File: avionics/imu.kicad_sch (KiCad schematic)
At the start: 3 parts, among them U2 BMI088

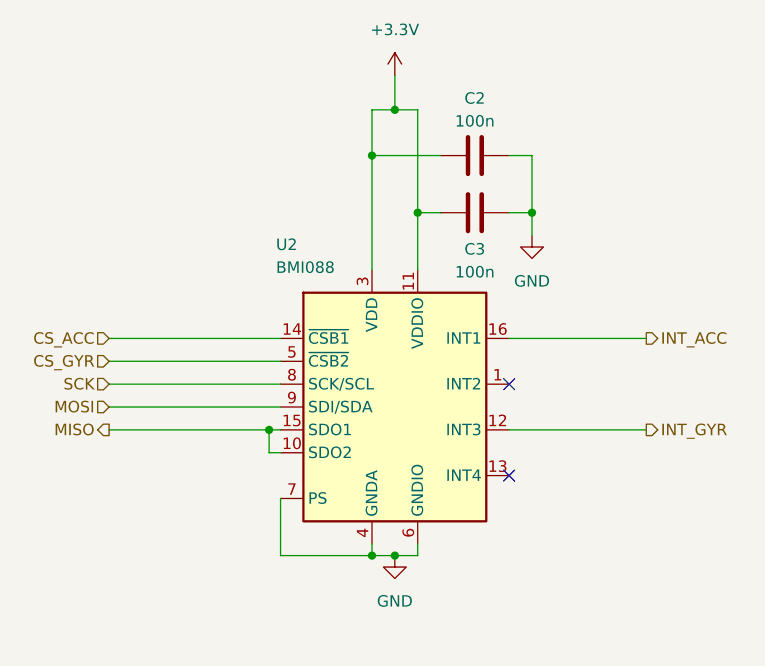
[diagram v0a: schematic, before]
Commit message: hw: order pcb
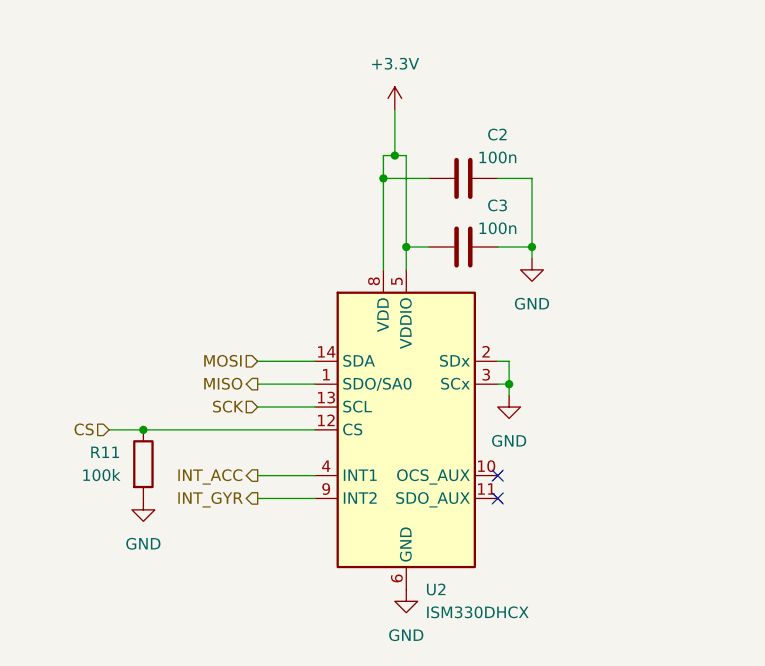
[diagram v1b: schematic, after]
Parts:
- removed U2: BMI088, libraries:PQFN50P450X300X100-16N, symbol Sensor_Motion:BMI088
- added R11: 100k, Resistor_SMD:R_0603_1608Metric, symbol Device:R
- added U2: ISM330DHCX, Package_LGA:LGA-14_3x2.5mm_P0.5mm_LayoutBorder3x4y, symbol Sensor_Motion:ISM330DHCX
- C2, C3: DigiKey Part Number (none) -> 399-C0603C104K5RACTUCT-ND
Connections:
- net +3.3V: now also C3.2, U2.5 (VDDIO), U2.8 (VDD); no longer C3.1
- net GND: now also C3.1, R11.2, U2.2 (SDx), U2.3 (SCx), U2.6 (GND), U2.7 (GND); no longer C3.2
- net INT_ACC: now also U2.4 (INT1)
- net INT_GYR: now also U2.9 (INT2)
- net MISO: now also U2.1 (SDO/SA0)
- net MOSI: now also U2.14 (SDA)
- net SCK: now also U2.13 (SCL)
- new net CS: R11.1, U2.12 (CS)
